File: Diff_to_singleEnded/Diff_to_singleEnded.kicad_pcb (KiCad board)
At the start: 6 copper layers, 85 x 65 mm, 46 parts, among them J1 Conn_01x01_Pin, J2 Conn_01x03_Socket, J3 1725672, J4 1725672, J5 1725672, U1 OPA1692xD, U2 OPA1692xD, U3 OPA1692xD

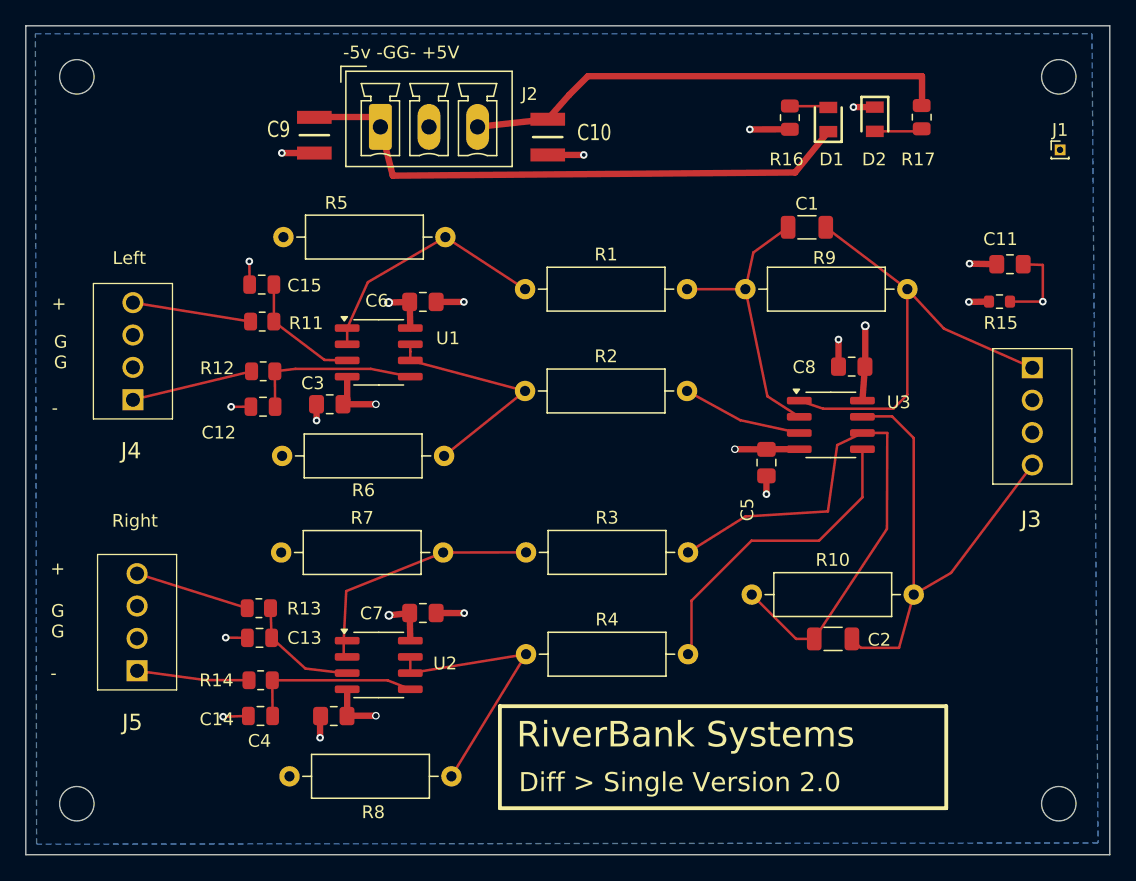
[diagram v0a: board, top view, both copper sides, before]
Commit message: add updates to se to diff
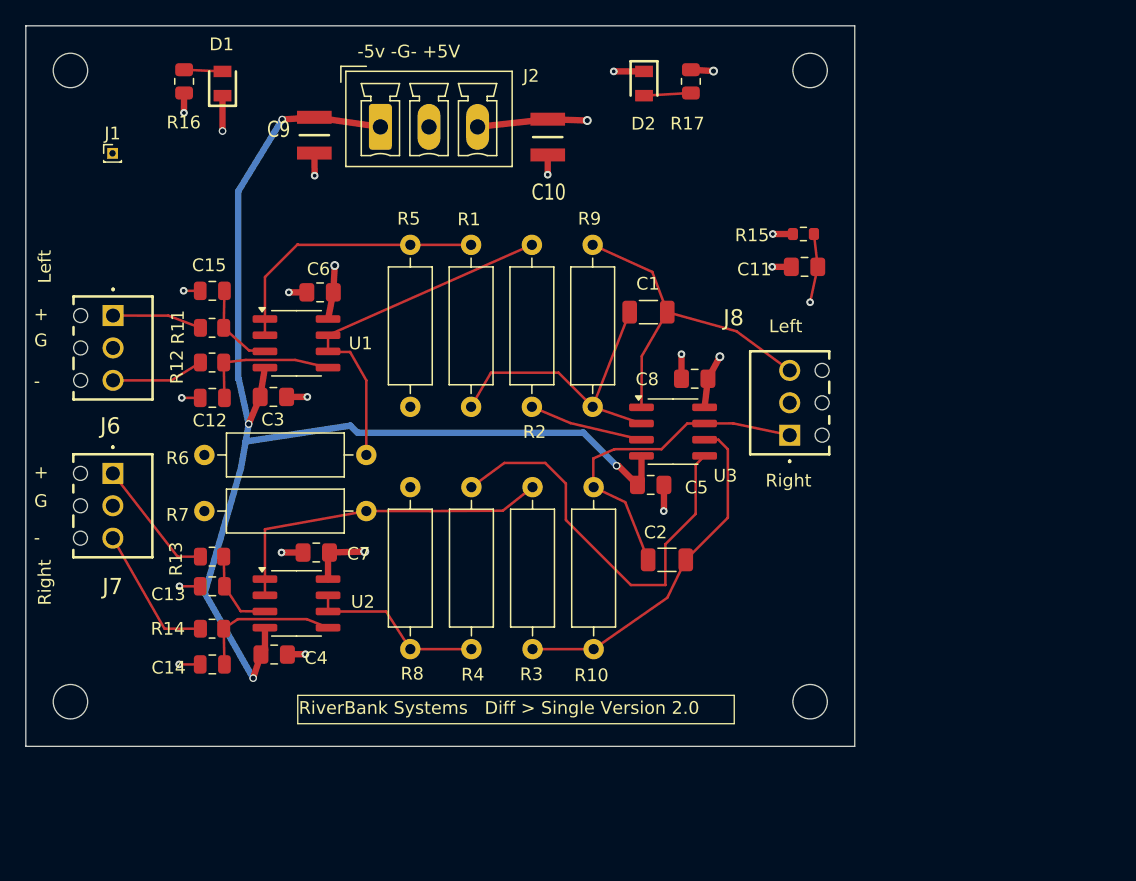
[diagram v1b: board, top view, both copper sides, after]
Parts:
- removed J3, J4, J5: 1725672, samsys:1725672
- added J6: 1725669, samsys:1725669, F.Cu at (106.8, 72.7)
- added J7: 1725669, samsys:1725669, F.Cu at (106.8, 85.1)
- added J8: 1725669, samsys:1725669, F.Cu at (159.9, 82.1)
- moved J1 74.3 mm to (106.8, 60.0)
- moved R16 47.6 mm to (112.4, 54.4)
- moved D1 47.6 mm to (115.4, 54.5)
- moved R8 24.6 mm to (130.2, 86.2), turned to -90 degrees
- moved H4 21.1 mm to (161.5, 103.0)
- moved H3 19.5 mm to (161.5, 53.5)
- moved R17 18.3 mm to (152.2, 54.4)
- moved D2 18.3 mm to (148.5, 54.5)
- moved R15 16.3 mm to (161.0, 66.3)
- moved C11 16.1 mm to (161.1, 68.9)
- moved R9 15.1 mm to (144.4, 79.9), turned to 90 degrees
- moved C2 14.4 mm to (150.3, 91.9), turned to 180 degrees
- moved C1 14.1 mm to (148.8, 72.5)
- moved R10 13.1 mm to (144.5, 98.9), turned to 90 degrees
- moved U3 12.4 mm to (150.8, 81.8)
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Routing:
- net -5V: track 150.7 -> 105.6 mm, vias 3 -> 5
- net +5V: track 160.3 -> 138.3 mm, vias 3 -> 5
- net Net-(U3B--): track 45.8 -> 27.3 mm
- net /Rout: track 39.3 -> 26.4 mm
- net Net-(U1B--): track 18.7 -> 28.9 mm
- net /Lout: track 37.1 -> 27.3 mm
- net Net-(U3B-+): track 24.8 -> 32.9 mm
- net Net-(U2B--): track 21.7 -> 14.1 mm
- net Net-(U2A--): track 19.8 -> 26.9 mm
- net GND: track 24.8 -> 20.5 mm
- net /buffer L- in: track 9.66 -> 6.81 mm
- net GND 2: track 14.0 -> 11.5 mm
- net /buffer L+: track 13.5 -> 11.0 mm
- net /buffer R+ in: track 13.8 -> 11.3 mm
- net /buffer R- in: track 8.93 -> 6.56 mm
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- added copper zone on In2.Cu, net GND
- added copper zone on In4.Cu, net GND 3
- removed copper zone on In3.Cu, net GND
- removed copper zone on B.Cu, net GND 3
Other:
- board size 85 x 65 mm -> 65 x 56.5 mm
- board text added: "-5v -G- +5V"
- board text added: "G"
- board text removed: "-5v -GG- +5V"
- board text removed: "G G"
